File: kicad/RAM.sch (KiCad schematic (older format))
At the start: 5 parts, among them U63 74LS08, U64 628128_DIP32_SSOP32, U65 74LS245, U66 74LS04, U67 28C256

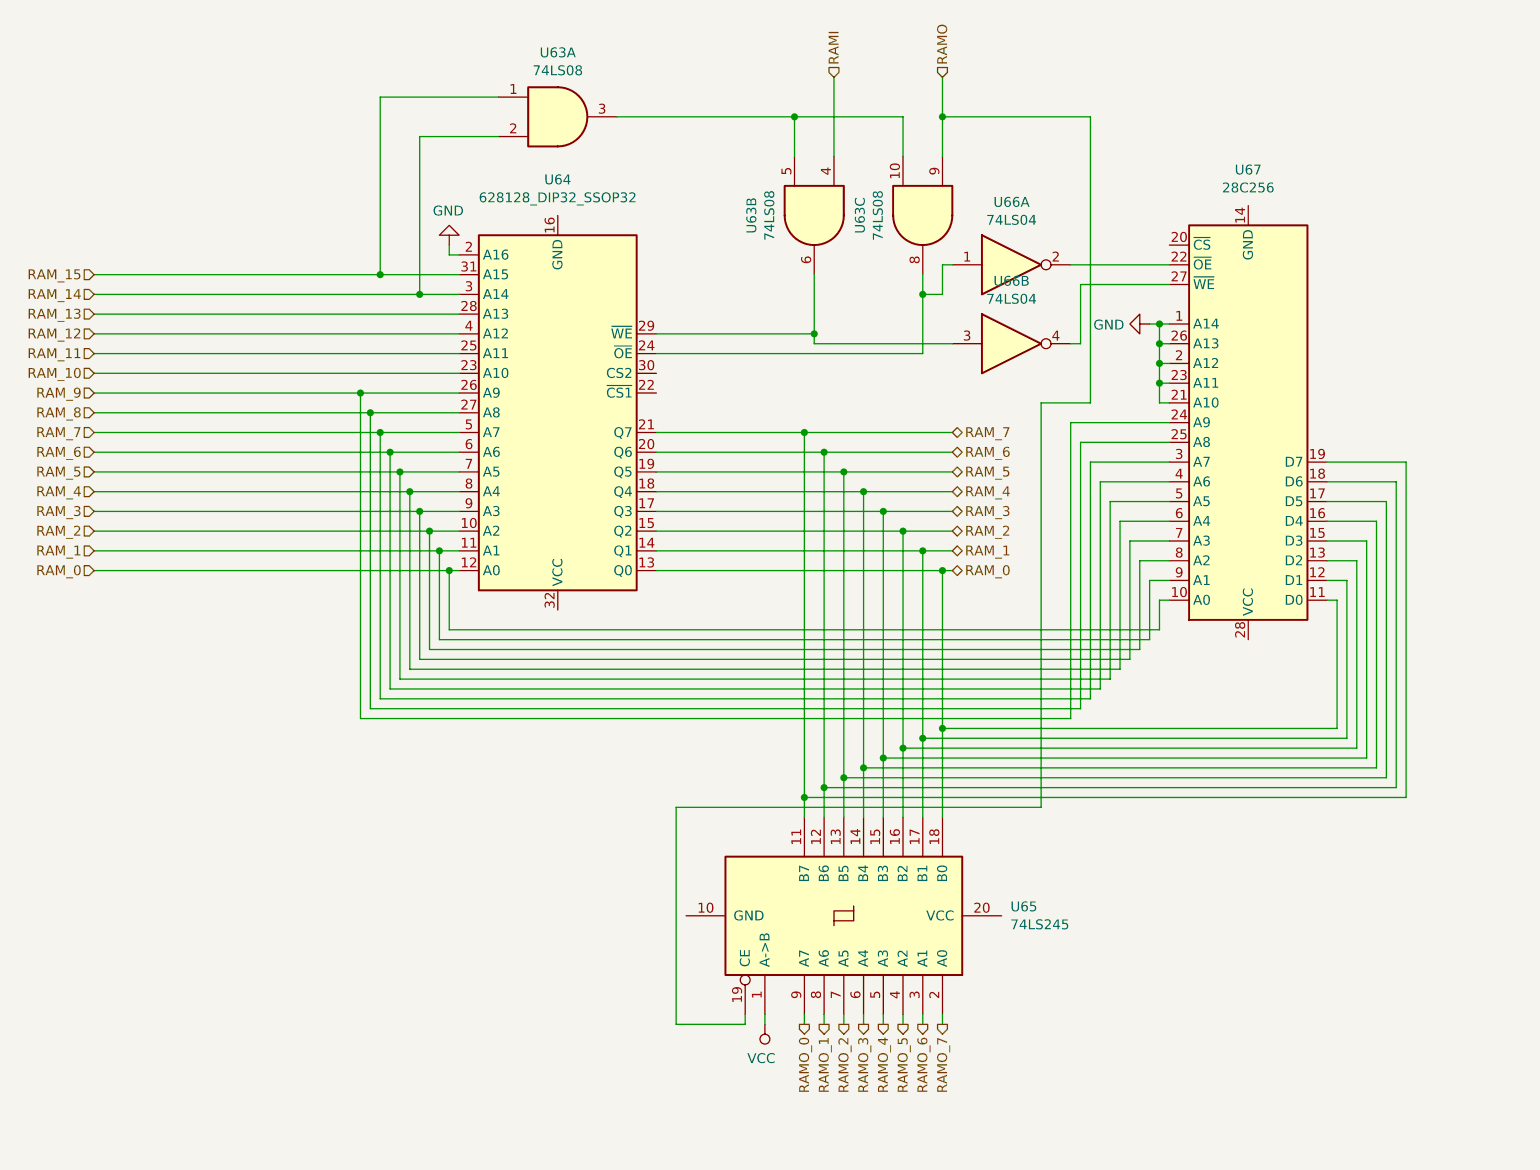
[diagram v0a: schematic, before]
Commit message: Up to v1.0 and plot
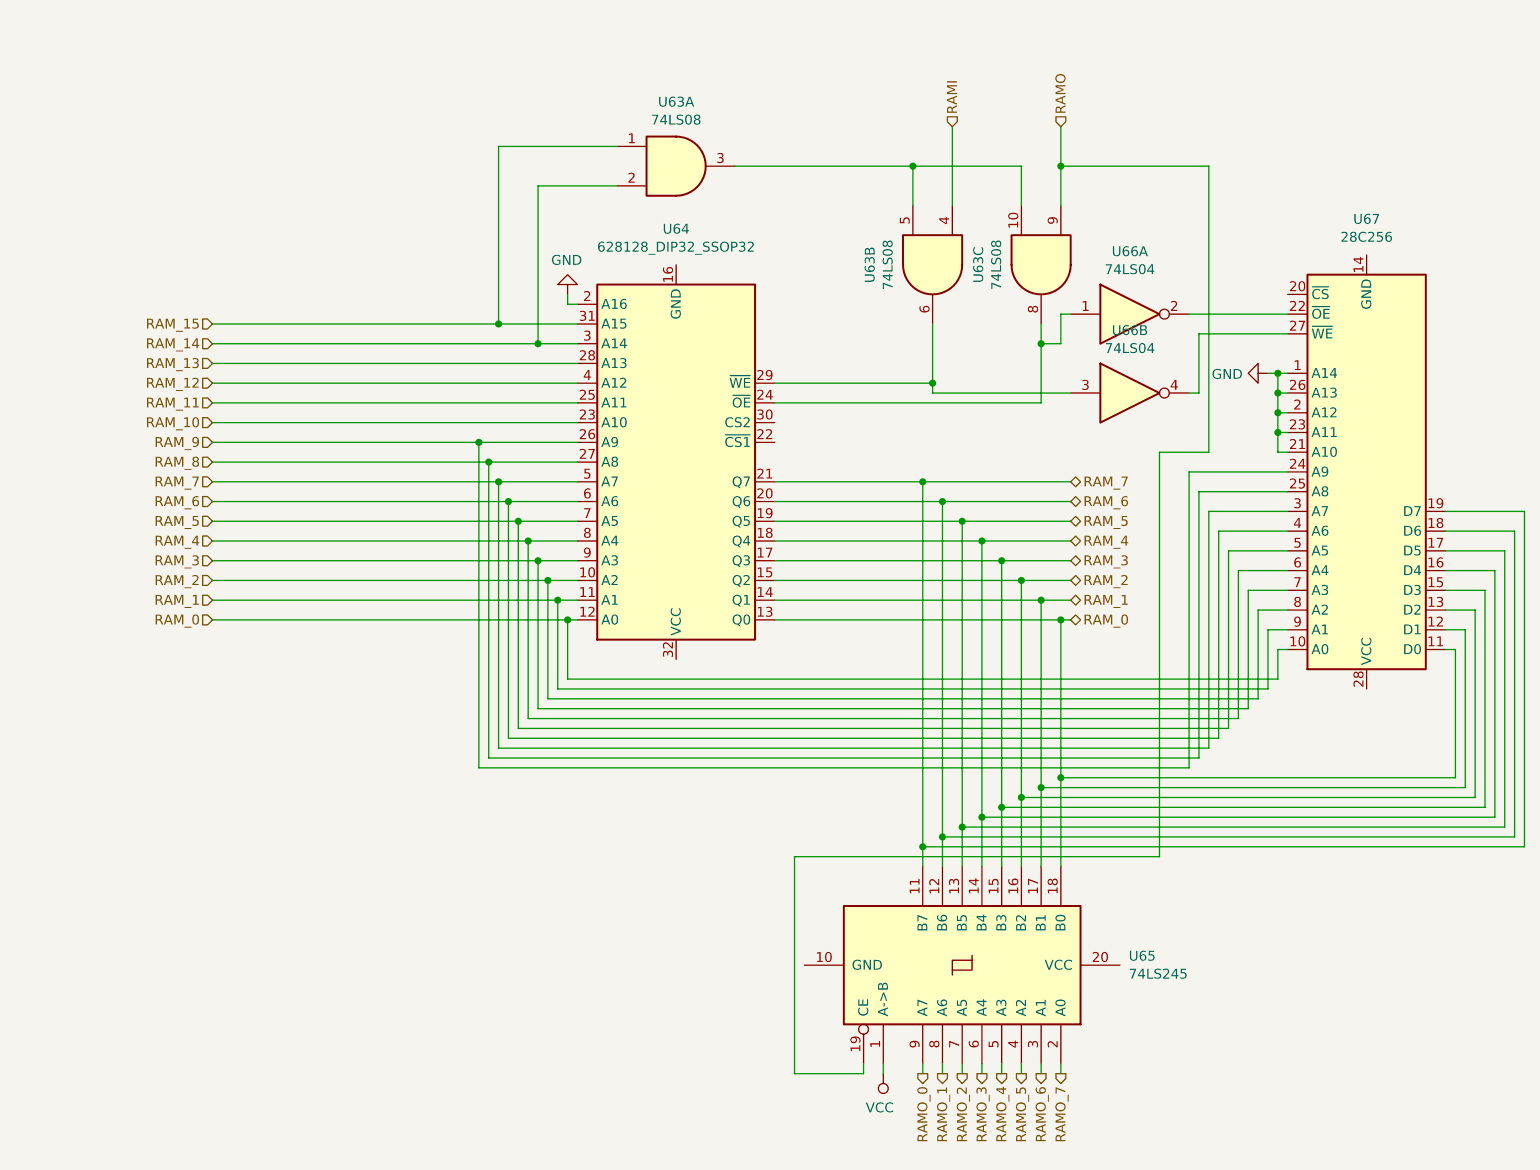
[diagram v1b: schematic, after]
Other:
- moved on the sheet: U63A, U63B, U63C, U64, U65, U66A, U66B, U67
